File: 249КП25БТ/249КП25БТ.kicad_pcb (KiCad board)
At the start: 2 copper layers, 15.5 x 13.8 mm, 5 parts

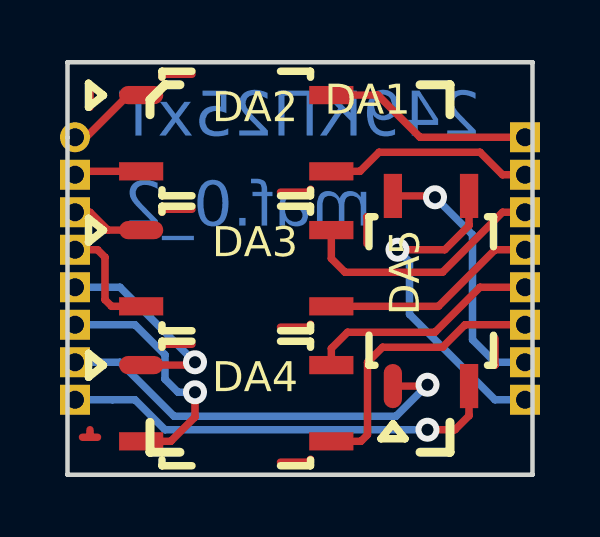
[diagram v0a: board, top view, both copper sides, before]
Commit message: Резонит плакал
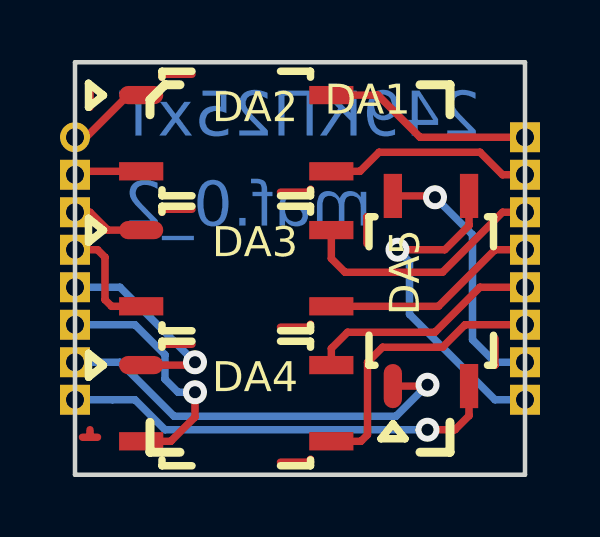
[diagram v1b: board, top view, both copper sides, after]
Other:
- board size 15.5 x 13.8 mm -> 15 x 13.8 mm
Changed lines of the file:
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@@
-(kicad_pcb (version 20171130) (host pcbnew "(5.0.0)")
+(kicad_pcb (version 20171130) (host pcbnew "(5.0.2)-1")
   (general
     (thickness 1.6)
-    (drawings 7)
+    (drawings 6)
     (tracks 106)
     (zones 0)
@@
       (drillshape 0)
       (scaleselection 1)
-      (outputdirectory "GERBER/maf_2/"))
+      (outputdirectory "maf_2/"))
   )
   (net 0 "")
@@
     (effects (font (size 1.5 1.5) (thickness 0.3)) (justify mirror))
   )
-  (gr_line (start 118.25 65.5) (end 118.25 68) (layer Edge.Cuts) (width 0.15))
-  (gr_line (start 133.75 65.5) (end 118.25 65.5) (layer Edge.Cuts) (width 0.15))
-  (gr_line (start 133.75 79.25) (end 133.75 65.5) (layer Edge.Cuts) (width 0.15))
-  (gr_line (start 118.25 79.25) (end 133.75 79.25) (layer Edge.Cuts) (width 0.15))
-  (gr_line (start 118.25 68) (end 118.25 79.25) (layer Edge.Cuts) (width 0.15))
+  (gr_line (start 133.5 65.5) (end 118.5 65.5) (layer Edge.Cuts) (width 0.15))
+  (gr_line (start 133.5 79.25) (end 133.5 65.5) (layer Edge.Cuts) (width 0.15))
+  (gr_line (start 118.5 79.25) (end 133.5 79.25) (layer Edge.Cuts) (width 0.15))
+  (gr_line (start 118.5 65.5) (end 118.5 79.25) (layer Edge.Cuts) (width 0.15))
   (segment (start 121.4 66) (end 121.4 65.90001) (width 0.25) (layer F.Cu) (net 0))
   (segment (start 121.4 65.90001) (end 122.39999 65.90001) (width 0.25) (layer F.Cu) (net 0))
